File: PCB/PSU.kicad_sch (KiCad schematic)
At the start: 48 parts, among them Q1 BSS138BKS, Q2 BSS138BKS, Q3 AO3401A, U12 TPS61040DBV, U13 INA180A4, U14 INA180A4, U6 AP2127K-ADJ, U7 AMS1117-3.3, U9 TPS259533

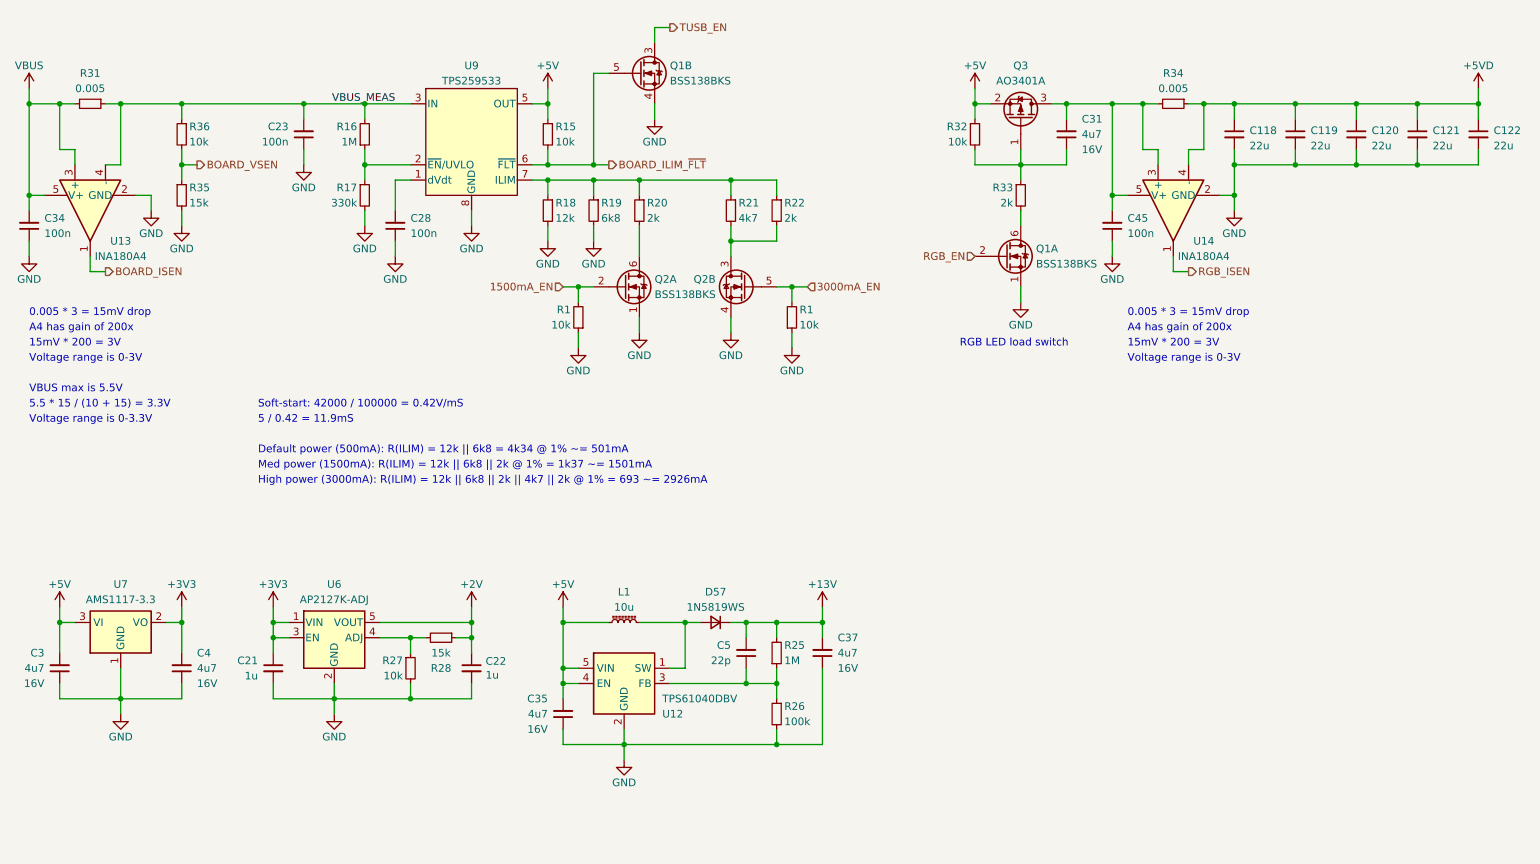
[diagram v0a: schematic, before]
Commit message: 05/05/2023 update.
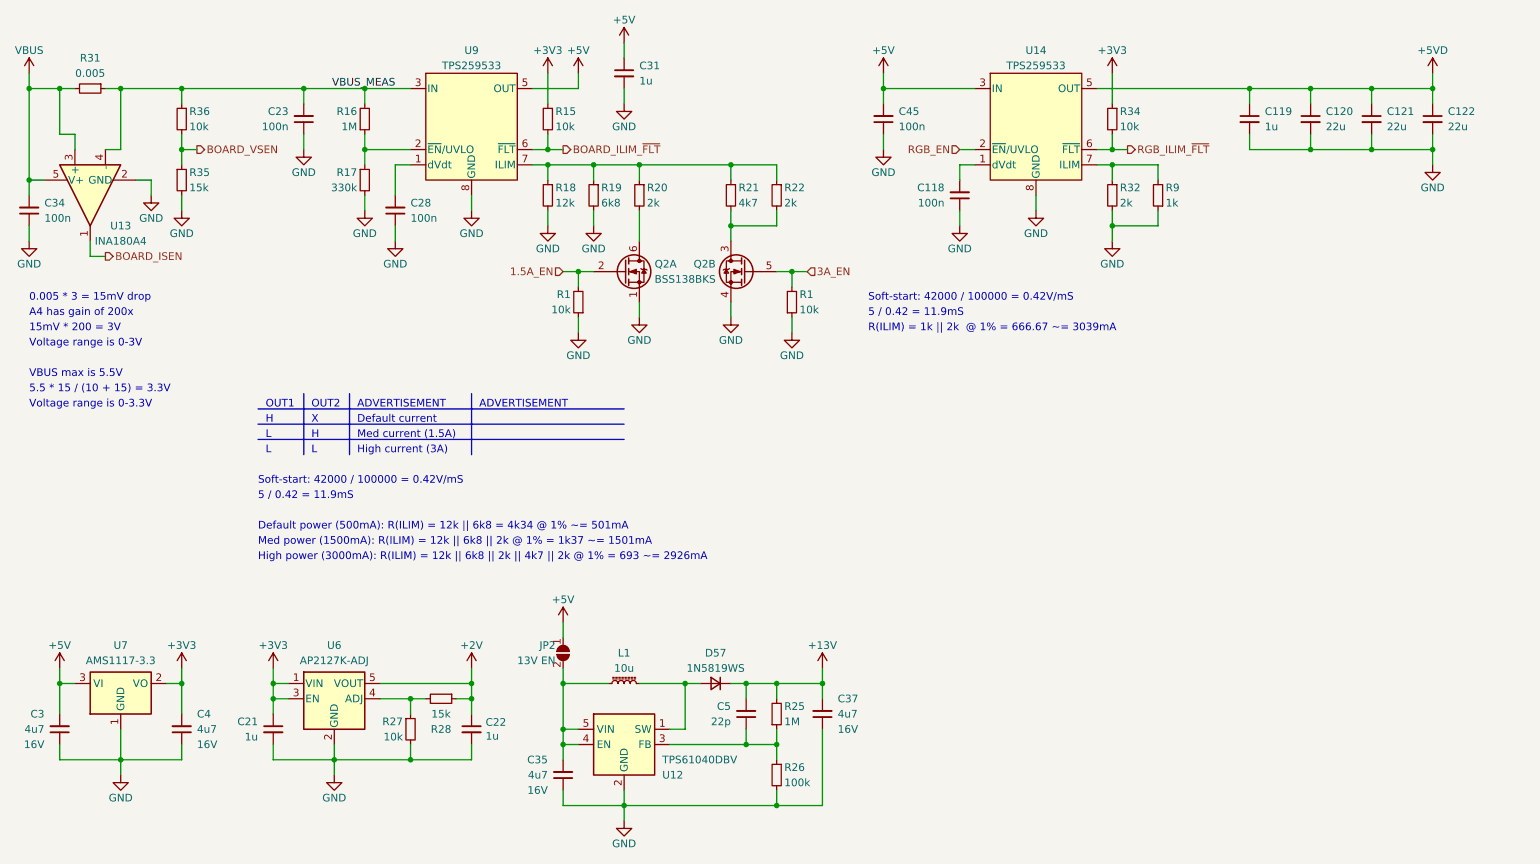
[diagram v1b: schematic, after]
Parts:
- removed Q1: BSS138BKS, Package_TO_SOT_SMD:SOT-363_SC-70-6, symbol Device:Q_Dual_NMOS_S1G1D2S2G2D1
- removed Q3: AO3401A, Package_TO_SOT_SMD:SOT-23, symbol Transistor_FET:AO3401A
- removed R33: 2k, Resistor_SMD:R_0402_1005Metric, symbol Device:R_Small
- removed U14: INA180A4, Package_TO_SOT_SMD:SOT-23-5, symbol Amplifier_Current:INA180A4
- added JP2: 13V EN, Honeydew:SolderJumper-2_P1.2mm_Open_Pad1.0x1.0mm, symbol Honeydew:SolderJumper_2_Open
- added R9: 1k, Resistor_SMD:R_0402_1005Metric, symbol Device:R_Small
- added U14: TPS259533, Honeydew:WSON-8-1EP_2x2mm_P0.5mm_EP0.9x1.6mm, symbol Honeydew:TPS259533
- C118: value 22u -> 100n; footprint Capacitor_SMD:C_0805_2012Metric -> Capacitor_SMD:C_0402_1005Metric; LCSC C45783 -> C307331; Voltage 25V -> 50V
- C119: value 22u -> 1u; footprint Capacitor_SMD:C_0805_2012Metric -> Capacitor_SMD:C_0603_1608Metric; LCSC C45783 -> C15849; Voltage 25V -> 50V
- C31: value 4u7 -> 1u; LCSC C19666 -> C15849; Voltage 16V -> 50V
- R32: value 10k -> 2k; LCSC C25744 -> C4109
- R34: value 0.005 -> 10k; footprint Resistor_SMD:R_0805_2012Metric -> Resistor_SMD:R_0402_1005Metric; LCSC C2939747 -> C25744
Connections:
- net +3V3: now also R15.1, R34.1
- net +5V: now also C31.1, C45.2, JP2.1 (A), U14.3 (IN), U14.4 (IN); no longer C35.2, L1.2, R15.1, R32.1, U12.4 (EN), U12.5 (VIN)
- net +5VD: now also U14.5 (OUT); no longer C118.1, R34.1
- net GND: now also C118.1, C31.2, R32.2, R9.1, U14.8 (GND), U14.9 (GND); no longer C118.2
- net RGB_EN: now also U14.2 (~{EN}/UVLO)
- net 1500mA_EN renamed 1.5A_EN
- net 3000mA_EN renamed 3A_EN
- new net: C35.2, JP2.2 (B), L1.2, U12.4 (EN), U12.5 (VIN)
- new net: C118.2, U14.1 (dVdt)
- new net: R32.1, R9.2, U14.7 (ILIM)
- new net RGB_ILIM_~{FLT}: R34.2, U14.6 (~{FLT})
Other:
- note added: "ADVERTISEMENT"
- note added: "Default current"
- note added: "H"
- note added: "High current (3A)"
- note added: "L"
- note added: "Med current (1.5A)"
- note added: "OUT1"
- note added: "OUT2"
- note added: "R(ILIM) = 1k || 2k @ 1% = 666.67 ~= 3039mA"
- note added: "X"
- note removed: "RGB LED load switch"
- moved on the sheet: C21, C22, C23, C28, C3, C34, C35, C37, C4, C5, D57, L1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
